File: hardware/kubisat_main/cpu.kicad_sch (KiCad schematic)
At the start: 8 parts, among them J2 Micro_SD_Card_Det1, J3 Conn_01x08_Socket, J4 Conn_01x08_Socket, J5 Conn_01x07_Socket

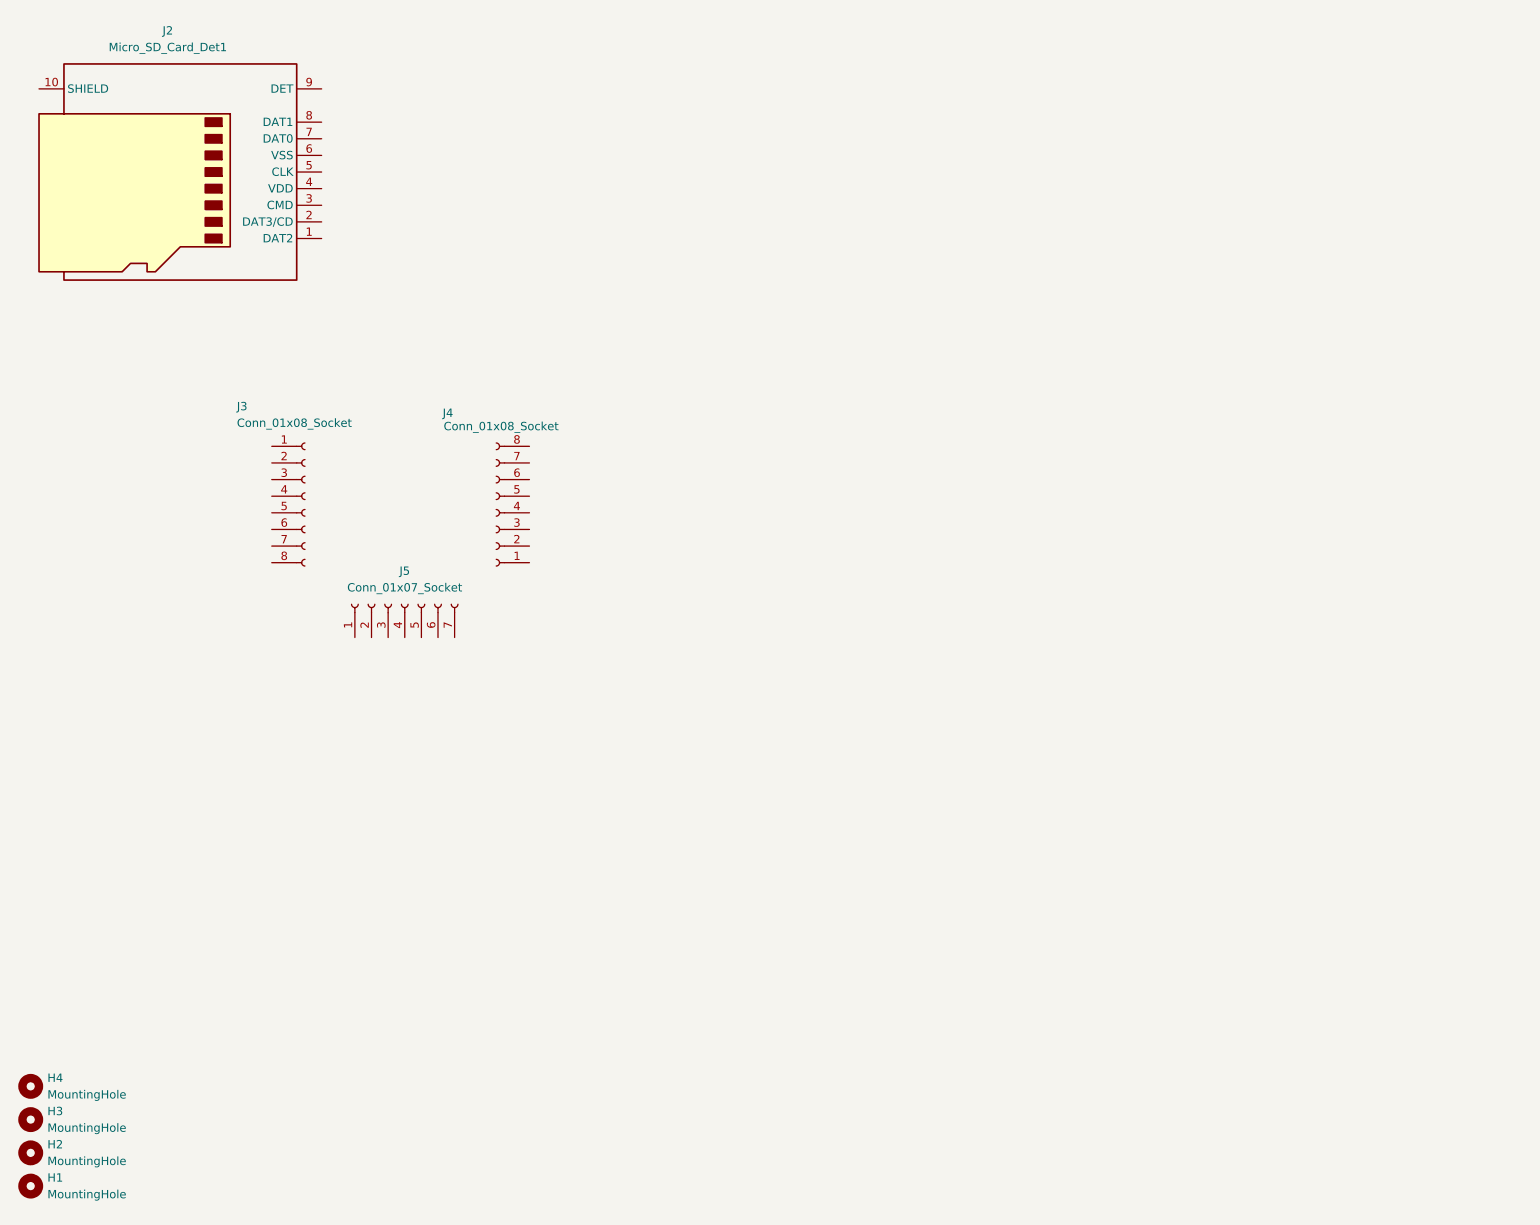
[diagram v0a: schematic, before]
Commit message: added elements to cpu schematic
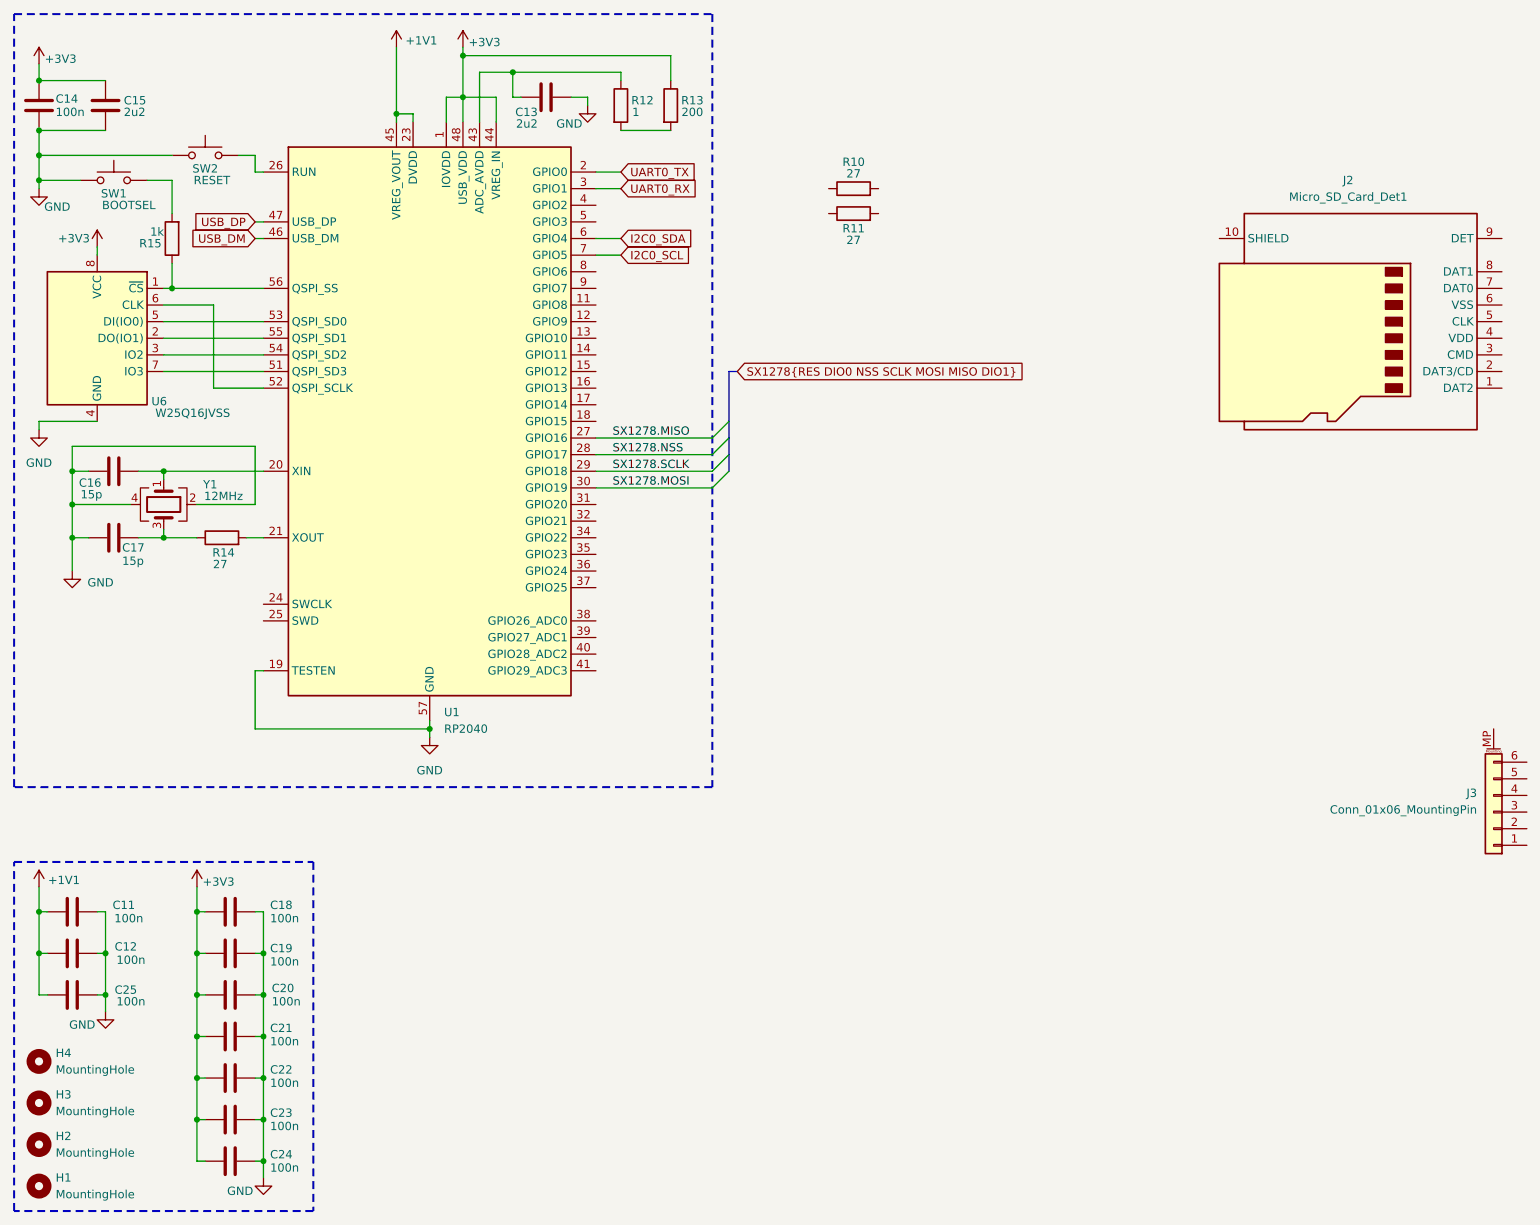
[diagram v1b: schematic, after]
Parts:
- removed J3, J4: Conn_01x08_Socket, Connector_PinHeader_2.54mm:PinHeader_1x08_P2.54mm_Vertical, symbol Connector:Conn_01x08_Socket
- removed J5: Conn_01x07_Socket, Connector_PinSocket_2.54mm:PinSocket_1x07_P2.54mm_Vertical, symbol Connector:Conn_01x07_Socket
- added C11, C12, C14, C18, C19, C20, C21, C22, C23, C24, C25: 100n, Capacitor_SMD:C_0805_2012Metric, symbol Device:C
- added C13, C15: 2u2, Capacitor_SMD:C_0805_2012Metric, symbol Device:C
- added C16, C17: 15p, Capacitor_SMD:C_0805_2012Metric, symbol Device:C
- added J3: Conn_01x06_MountingPin, Connector_JST:JST_PH_S6B-PH-SM4-TB_1x06-1MP_P2.00mm_Horizontal, symbol Connector_Generic_MountingPin:Conn_01x06_MountingPin
- added R10, R11, R14: 27, symbol Device:R
- added R12: 1, symbol Device:R
- added R13: 200, symbol Device:R
- added R15: 1k, symbol Device:R
- added SW1: BOOTSEL, Button_Switch_SMD:SW_MEC_5GSH9, symbol Switch:SW_Push
- added SW2: RESET, Button_Switch_SMD:SW_MEC_5GSH9, symbol Switch:SW_Push
- added U1: RP2040, Package_DFN_QFN:QFN-56-1EP_7x7mm_P0.4mm_EP3.2x3.2mm, symbol MCU_RaspberryPi:RP2040
- added U6: W25Q16JVSS, Package_SO:SOIC-8_5.23x5.23mm_P1.27mm, symbol Memory_Flash:W25Q16JVSS
- added Y1: 12MHz, Crystal:Crystal_SMD_3225-4Pin_3.2x2.5mm, symbol Device:Crystal_GND24
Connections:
- new net: C13.2, R12.1, U1.43 (ADC_AVDD)
- new net: R12.2, R13.2
- new net: R15.2, SW1.2
- new net: C17.2, R14.1, Y1.3
- new net: R14.2, U1.21 (XOUT)
- new net: C16.2, U1.20 (XIN), Y1.1
- new net: SW2.2, U1.26 (RUN)
- new net: U1.51 (QSPI_SD3), U6.7 (IO3)
- new net: U1.52 (QSPI_SCLK), U6.6 (CLK)
- new net: U1.53 (QSPI_SD0), U6.5 (DI(IO0))
- new net: U1.54 (QSPI_SD2), U6.3 (IO2)
- new net: U1.55 (QSPI_SD1), U6.2 (DO(IO1))
- new net: R15.1, U1.56 (QSPI_SS), U6.1 (~{CS})
- new net +1V1: C11.1, C12.2, C25.2, U1.23 (DVDD), U1.45 (VREG_VOUT), U1.50 (DVDD)
- new net +3V3: C14.2, C15.2, C18.1, C19.1, C20.1, C21.1, C22.1, C23.1, C24.1, R13.1, U1.1 (IOVDD), U1.10 (IOVDD), U1.22 (IOVDD), U1.33 (IOVDD), U1.42 (IOVDD), U1.44 (VREG_IN), U1.48 (USB_VDD), U1.49 (IOVDD), U6.8 (VCC)
- new net GND: C11.2, C12.1, C13.1, C14.1, C15.1, C16.1, C17.1, C18.2, C19.2, C20.2, C21.2, C22.2, C23.2, C24.2, C25.1, SW1.1, SW2.1, U1.19 (TESTEN), U1.57 (GND), U6.4 (GND), Y1.2, Y1.4
- new net I2C0_SCL: U1.7 (GPIO5)
- new net I2C0_SDA: U1.6 (GPIO4)
- new net SX1278.MISO: U1.27 (GPIO16)
- new net SX1278.MOSI: U1.30 (GPIO19)
- new net SX1278.NSS: U1.28 (GPIO17)
- new net SX1278.SCLK: U1.29 (GPIO18)
- new net UART0_RX: U1.3 (GPIO1)
- new net UART0_TX: U1.2 (GPIO0)
- new net USB_DM: U1.46 (USB_DM)
- new net USB_DP: U1.47 (USB_DP)
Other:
- moved on the sheet: H1, H2, H3, H4, J2
